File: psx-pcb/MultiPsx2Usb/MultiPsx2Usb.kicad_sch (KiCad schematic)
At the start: 4 parts, among them J1 AVR-UPDI-6

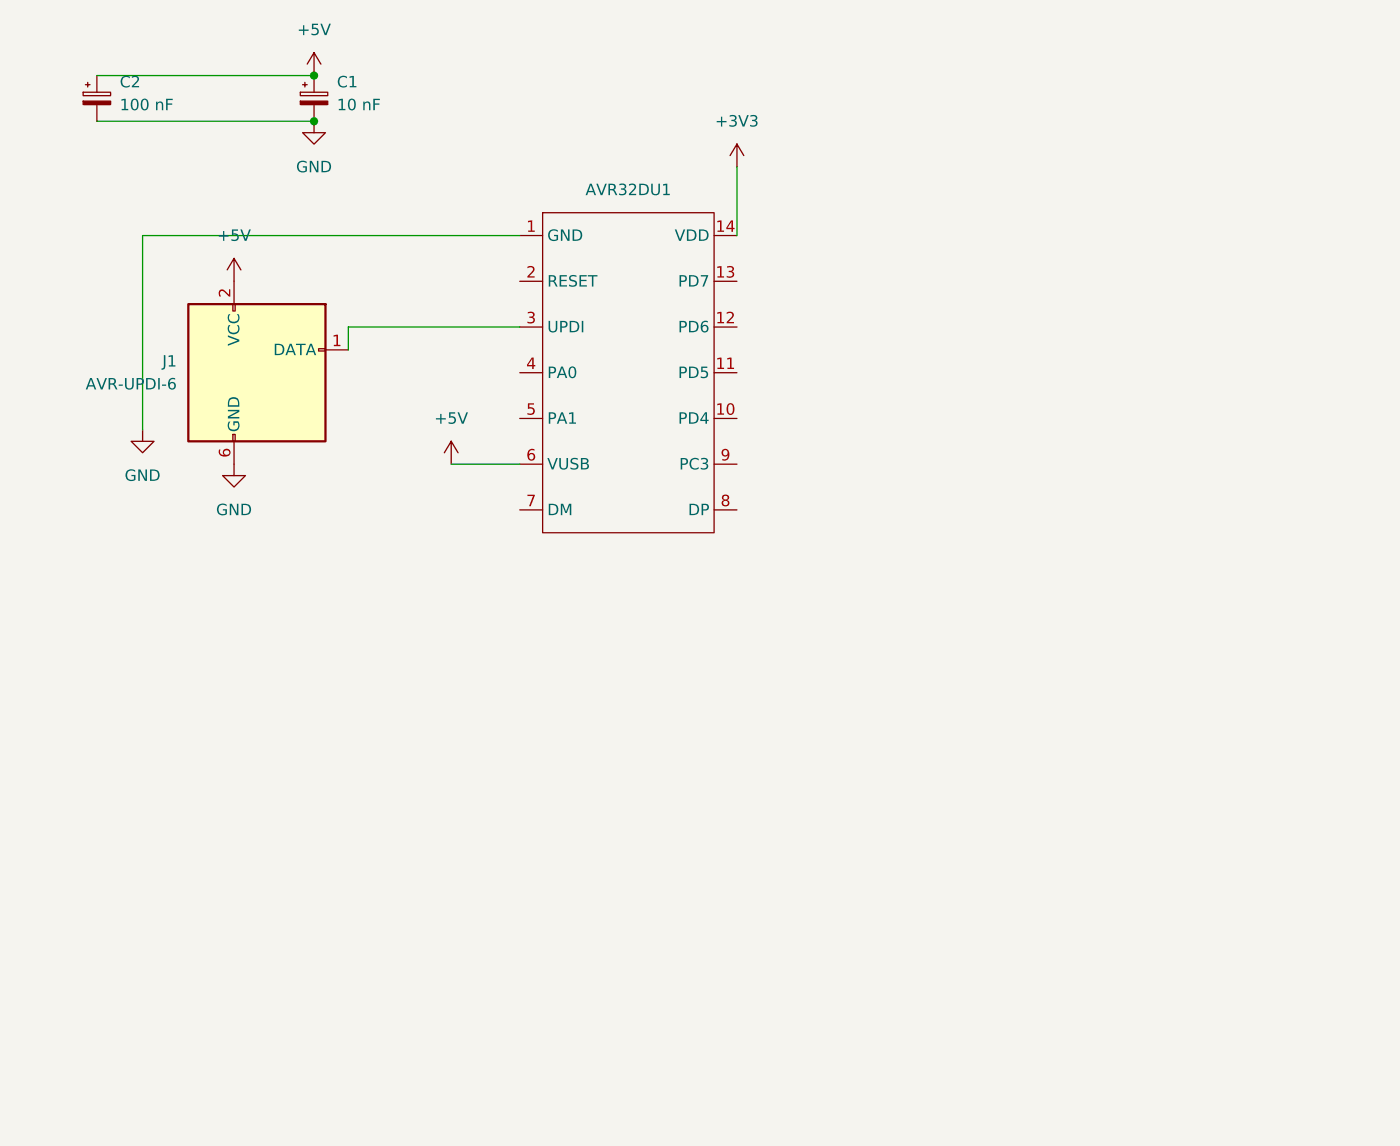
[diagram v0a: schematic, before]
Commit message: Rough schematic mockup done. need to create test circuits and see what works and what doesn't.
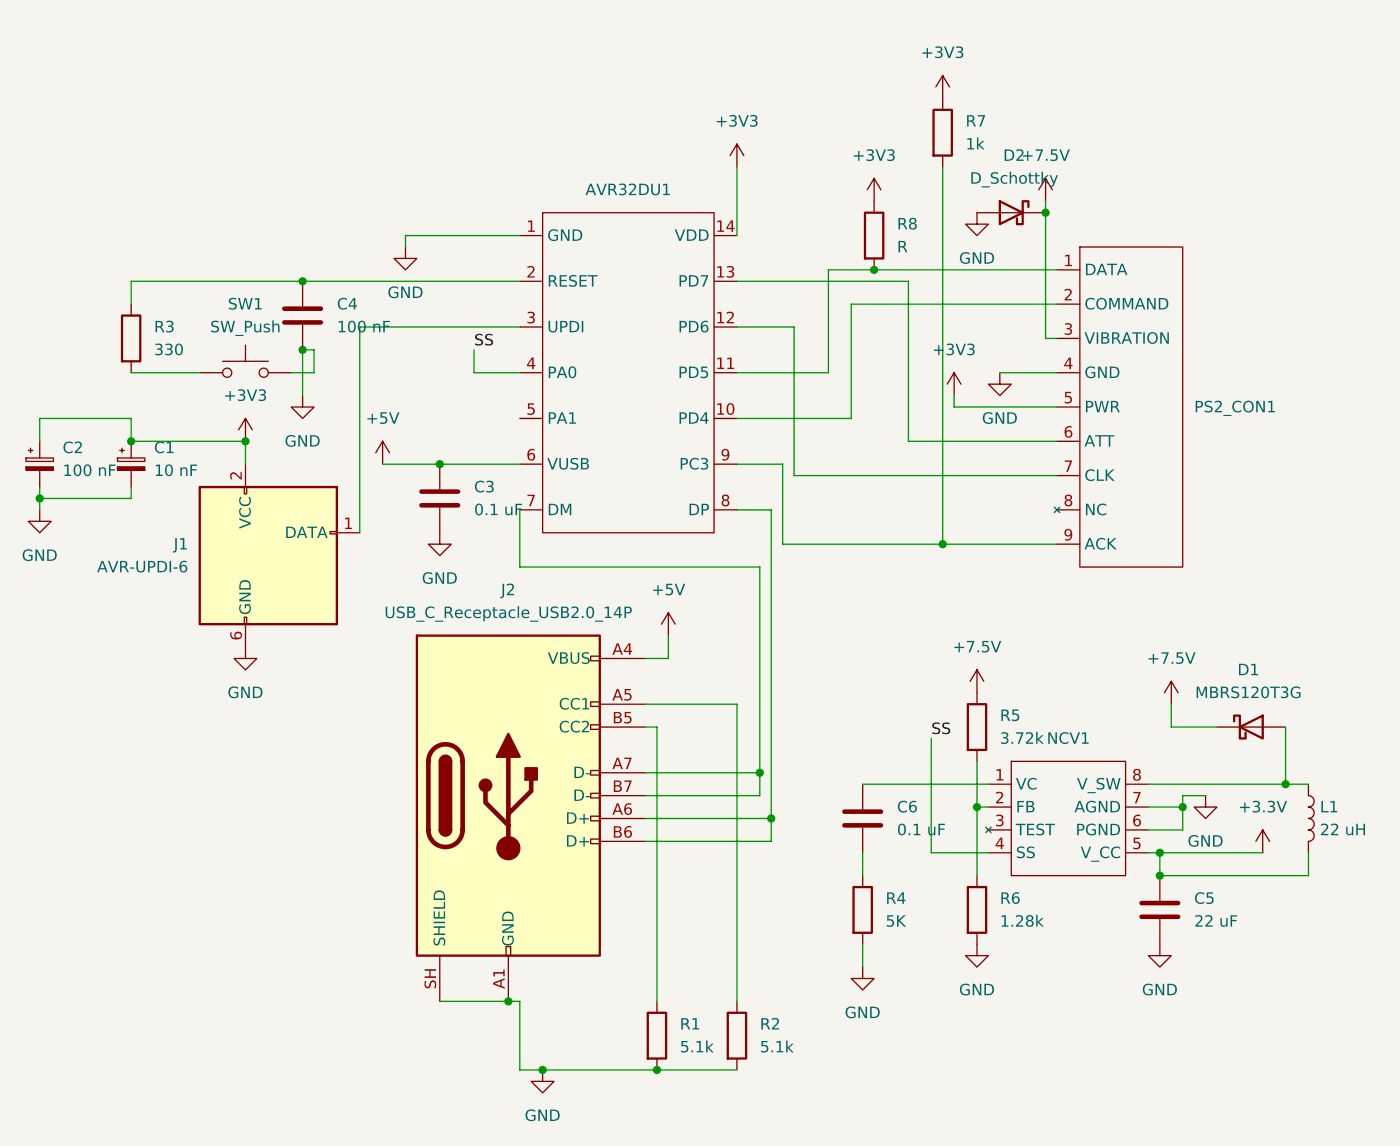
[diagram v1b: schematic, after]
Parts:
- added C3, C6: 0.1 uF, Capacitor_SMD:C_0603_1608Metric_Pad1.08x0.95mm_HandSolder, symbol Device:C
- added C4: 100 nF, Capacitor_SMD:C_0603_1608Metric_Pad1.08x0.95mm_HandSolder, symbol Device:C
- added C5: 22 uF, Capacitor_SMD:C_0603_1608Metric_Pad1.08x0.95mm_HandSolder, symbol Device:C
- added D1: MBRS120T3G, Diode_SMD:D_SMB_Handsoldering, symbol Device:D_Schottky
- added D2: D_Schottky, symbol Device:D_Schottky
- added J2: USB_C_Receptacle_USB2.0_14P, symbol Connector:USB_C_Receptacle_USB2.0_14P
- added L1: 22 uH, Inductor_SMD:L_0603_1608Metric_Pad1.05x0.95mm_HandSolder, symbol Device:L
- added NCV1: (no value), Package_SO:SOIC-8-1EP_3.9x4.9mm_P1.27mm_EP2.41x3.81mm_ThermalVias, symbol avr32du:NCV5171
- added PS2_CON1: (no value), avr32du:PS2_CONNECTOR, symbol avr32du:PS2_CONNECTOR
- added R1, R2: 5.1k, Resistor_SMD:R_0603_1608Metric_Pad0.98x0.95mm_HandSolder, symbol Device:R
- added R3: 330, Resistor_SMD:R_0603_1608Metric_Pad0.98x0.95mm_HandSolder, symbol Device:R
- added R4: 5K, Resistor_SMD:R_0603_1608Metric_Pad0.98x0.95mm_HandSolder, symbol Device:R
- added R5: 3.72k, Resistor_SMD:R_0603_1608Metric_Pad0.98x0.95mm_HandSolder, symbol Device:R
- added R6: 1.28k, Resistor_SMD:R_0603_1608Metric_Pad0.98x0.95mm_HandSolder, symbol Device:R
- added R7: 1k, Resistor_SMD:R_0603_1608Metric_Pad0.98x0.95mm_HandSolder, symbol Device:R
- added R8: R, Resistor_SMD:R_0603_1608Metric_Pad0.98x0.95mm_HandSolder, symbol Device:R
- added SW1: SW_Push, Button_Switch_SMD:SW_Push_1P1T_XKB_TS-1187A, symbol Switch:SW_Push
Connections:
- net +3V3: now also C1.1, C2.1, J1.2 (VCC), PS2_CON1.5 (PWR), R7.1, R8.1
- net +5V: now also C3.1, J2.A4 (VBUS), J2.A9 (VBUS), J2.B4 (VBUS), J2.B9 (VBUS); no longer C1.1, C2.1, J1.2 (VCC)
- net GND: now also C3.2, C4.2, C5.2, D2.2 (A), J2.A1 (GND), J2.A12 (GND), J2.B1 (GND), J2.B12 (GND), J2.SH (SHIELD), NCV1.6 (PGND), NCV1.7 (AGND), PS2_CON1.4 (GND), R1.2, R2.2, R4.2, R6.2, SW1.2
- net at AVR32DU1.10 (PD4): now also PS2_CON1.2 (COMMAND)
- net at AVR32DU1.11 (PD5): now also PS2_CON1.1 (DATA), R8.2
- net at AVR32DU1.12 (PD6): now also PS2_CON1.7 (CLK)
- net at AVR32DU1.13 (PD7): now also PS2_CON1.6 (ATT)
- net at AVR32DU1.2 (RESET): now also C4.1, R3.1
- net SS: now reaches AVR32DU1.4 (PA0)
- net SS: now also NCV1.4 (SS)
- net at AVR32DU1.7 (DM): now also J2.A7 (D-), J2.B7 (D-)
- net at AVR32DU1.8 (DP): now also J2.A6 (D+), J2.B6 (D+)
- net at AVR32DU1.9 (PC3): now also PS2_CON1.9 (ACK), R7.2
- new net: J2.A5 (CC1), R2.1
- new net: C6.1, NCV1.1 (VC)
- new net: C6.2, R4.1
- new net: NCV1.2 (FB), R5.2, R6.1
- new net: J2.B5 (CC2), R1.1
- new net: D1.2 (A), L1.1, NCV1.8 (V_SW)
- new net: R3.2, SW1.1
- new net +3.3V: C5.1, L1.2, NCV1.5 (V_CC)
- new net +7.5V: D1.1 (K), D2.1 (K), PS2_CON1.3 (VIBRATION), R5.1
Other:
- moved on the sheet: C1, C2, J1
